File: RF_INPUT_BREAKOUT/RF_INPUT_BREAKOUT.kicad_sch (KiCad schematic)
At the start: 18 parts, among them IC1 SI4705-D62-GM, J1 5V Input, J2 I2C, J3 I2C, U1 LD1117S33TR_SOT223, U2 LT5512EUF-PBF, U3 Si5351A-B-GT

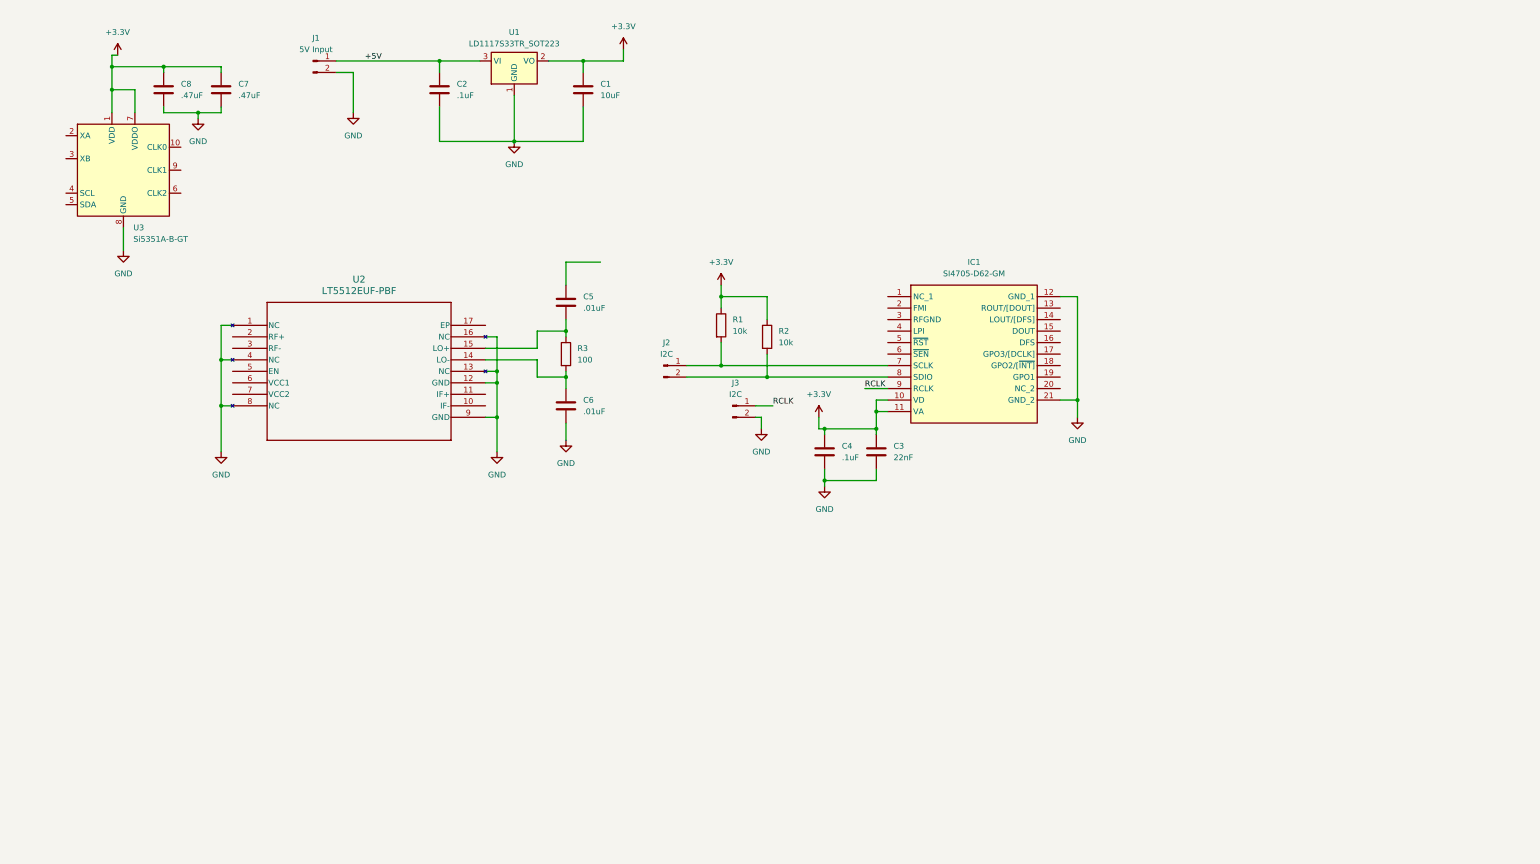
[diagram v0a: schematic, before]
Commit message: Did added external osc
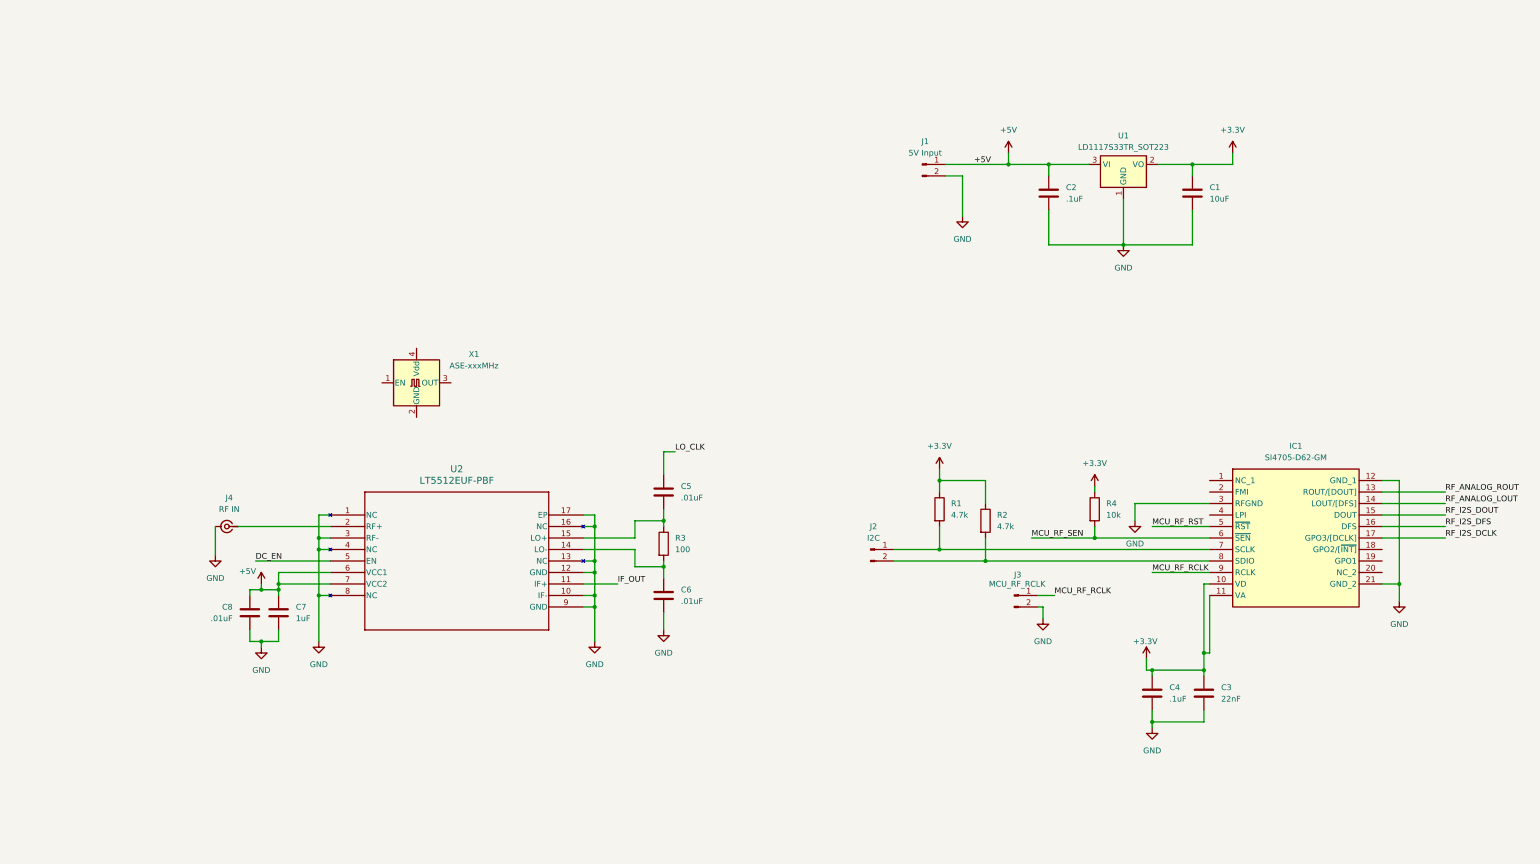
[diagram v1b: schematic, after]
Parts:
- removed U3: Si5351A-B-GT, Package_SO:MSOP-10_3x3mm_P0.5mm, symbol Oscillator:Si5351A-B-GT
- added J4: RF IN, symbol Connector:Conn_Coaxial_Small
- added R4: 10k, symbol Device:R
- added X1: ASE-xxxMHz, Oscillator:Oscillator_SMD_Abracon_ASE-4Pin_3.2x2.5mm, symbol Oscillator:ASE-xxxMHz
- C7: value .47uF -> 1uF
- C8: value .47uF -> .01uF
- J3: value I2C -> MCU_RF_RCLK
- R1, R2: value 10k -> 4.7k
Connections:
- net +3.3V: now also R4.1; no longer C7.1, C8.1
- net +5V: now also C7.1, C8.1, U2.6 (VCC1), U2.7 (VCC2)
- net GND: now also IC1.3 (RFGND), U2.10 (IF-), U2.17 (EP), U2.3 (RF-), J4.2 (Ext)
- net IF_OUT: now reaches U2.11 (IF+)
- net at U2.2 (RF+): now also J4.1 (In)
- net DC_EN: now reaches U2.5 (EN)
- net LO_CLK: now reaches C5.1
- net RF_ANALOG_ROUT: now reaches IC1.13 (ROUT/[DOUT])
- net RF_ANALOG_LOUT: now reaches IC1.14 (LOUT/[DFS])
- net RF_I2S_DOUT: now reaches IC1.15 (DOUT)
- net RF_I2S_DFS: now reaches IC1.16 (DFS)
- net RF_I2S_DCLK: now reaches IC1.17 (GPO3/[DCLK])
- net MCU_RF_RST: now reaches IC1.5 (~{RST})
- net MCU_RF_SEN: now reaches IC1.6 (~{SEN})
- net MCU_RF_SEN: now also R4.2
- net RCLK renamed MCU_RF_RCLK
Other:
- moved on the sheet: C1, C2, C3, C4, C5, C6, IC1, J1, J2, J3, R1, R2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

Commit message: added headers
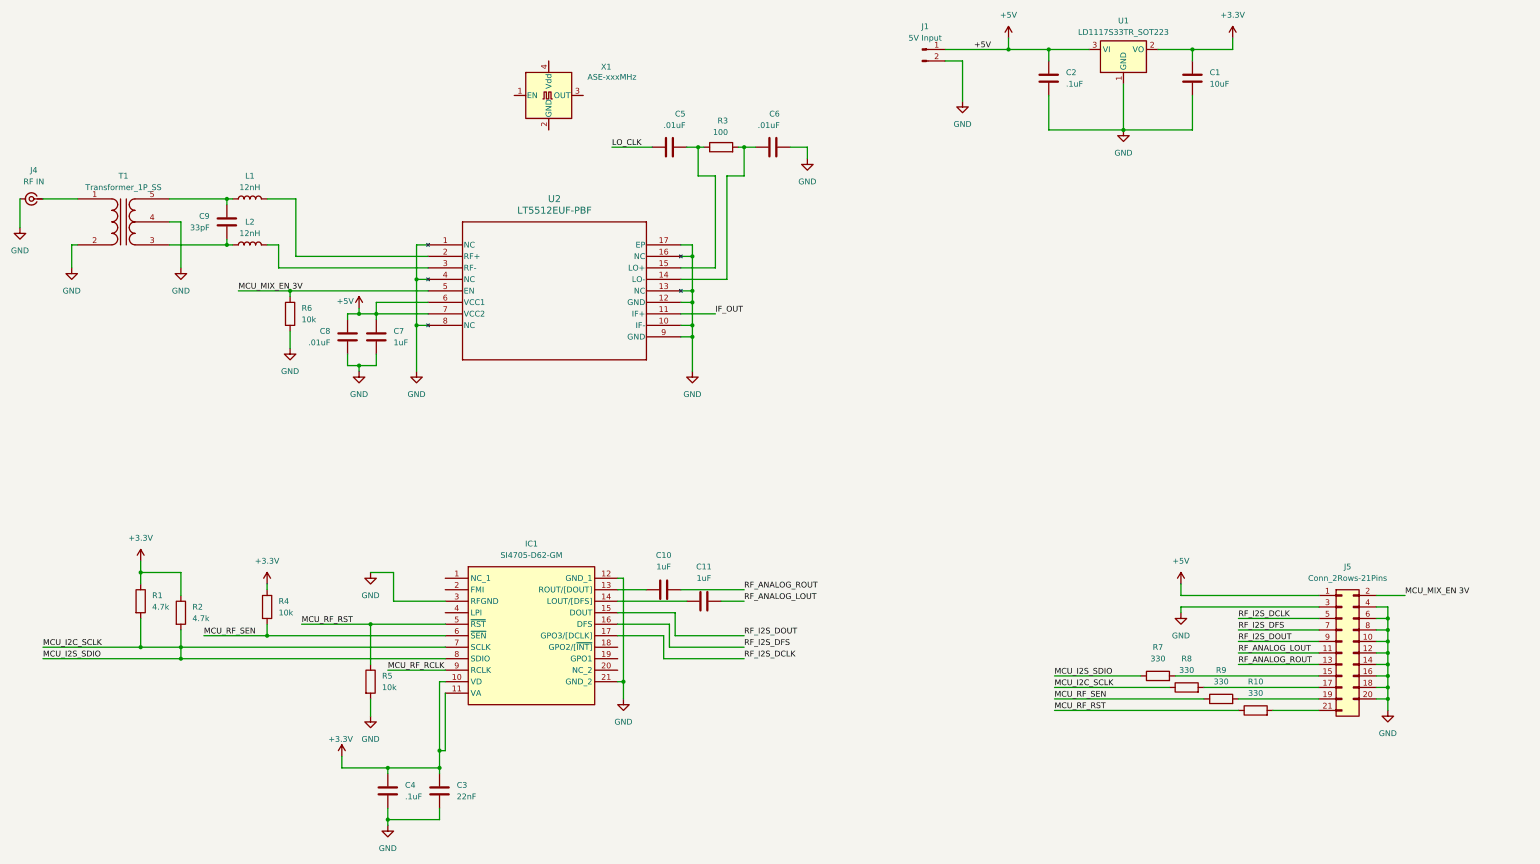
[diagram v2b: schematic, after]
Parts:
- removed J2: I2C, symbol Connector:Conn_01x02_Pin
- removed J3: MCU_RF_RCLK, symbol Connector:Conn_01x02_Pin
- added C10, C11: 1uF, Capacitor_SMD:C_0402_1005Metric, symbol Device:C
- added C9: 33pF, Capacitor_SMD:C_0402_1005Metric, symbol Device:C
- added J5: Conn_2Rows-21Pins, Connector_PinHeader_1.00mm:PinHeader_2x11_P1.00mm_Vertical, symbol Connector_Generic:Conn_2Rows-21Pins
- added L1, L2: 12nH, Inductor_SMD:L_0402_1005Metric, symbol Device:L
- added R10, R7, R8, R9: 330, Resistor_SMD:R_0402_1005Metric, symbol Device:R
- added R5, R6: 10k, Resistor_SMD:R_0402_1005Metric, symbol Device:R
- added T1: Transformer_1P_SS, symbol Device:Transformer_1P_SS
- C1: footprint (none) -> Capacitor_SMD:C_1206_3216Metric
- C2, C7: footprint (none) -> Capacitor_SMD:C_0201_0603Metric
- C3, C4, C5, C6, C8: footprint (none) -> Capacitor_SMD:C_0402_1005Metric
- IC1: footprint SI4705D62GM -> Package_DFN_QFN:QFN-20-1EP_3x3mm_P0.4mm_EP1.65x1.65mm
- R1, R2, R3, R4: footprint (none) -> Resistor_SMD:R_0402_1005Metric
- U2: footprint QFN-16_UF_LIT -> Package_DFN_QFN:QFN-16-1EP_4x4mm_P0.5mm_EP2.45x2.45mm
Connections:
- net +5V: now also J5.1 (Pin_1)
- net GND: now also J5.10 (Pin_10), J5.12 (Pin_12), J5.14 (Pin_14), J5.16 (Pin_16), J5.18 (Pin_18), J5.20 (Pin_20), J5.3 (Pin_3), J5.4 (Pin_4), J5.6 (Pin_6), J5.8 (Pin_8), R5.2, R6.2, T1.2 (AB), T1.4 (SC); no longer U2.3 (RF-)
- net MCU_RF_RST: now also R10.1, R5.1
- net MCU_RF_SEN: now also R9.1
- net RF_ANALOG_LOUT: now also C11.1, J5.11 (Pin_11); no longer IC1.14 (LOUT/[DFS])
- net RF_ANALOG_ROUT: now also C10.1, J5.13 (Pin_13); no longer IC1.13 (ROUT/[DOUT])
- net RF_I2S_DCLK: now also J5.5 (Pin_5)
- net RF_I2S_DFS: now also J5.7 (Pin_7)
- net RF_I2S_DOUT: now also J5.9 (Pin_9)
- net at U2.2 (RF+): now also L1.2; no longer J4.1 (In)
- net MCU_I2C_SCLK: now reaches IC1.8 (SDIO), R2.2
- net MCU_I2C_SCLK: now also IC1.7 (SCLK), R1.2, R7.1, R8.1
- net DC_EN renamed MCU_MIX_EN 3V
- net MCU_MIX_EN 3V: now also J5.2 (Pin_2), R6.1
- new net: C11.2, IC1.14 (LOUT/[DFS])
- new net: L2.2, U2.3 (RF-)
- new net: J4.1 (In), T1.1 (AA)
- new net: C10.2, IC1.13 (ROUT/[DOUT])
- new net: C9.1, L1.1, T1.5 (SB)
- new net: J5.15 (Pin_15), R7.2
- new net: C9.2, L2.1, T1.3 (SA)
- new net: J5.19 (Pin_19), R9.2
- new net: J5.17 (Pin_17), R8.2
- new net: J5.21 (Pin_21), R10.2
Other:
- moved on the sheet: C1, C2, C3, C4, C5, C6, C7, C8, IC1, J1, J4, R1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
